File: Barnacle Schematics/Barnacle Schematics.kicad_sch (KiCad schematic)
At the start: 17 parts, among them M3 MG996, M4 SG90, SW1 Reset, U1 TiVa

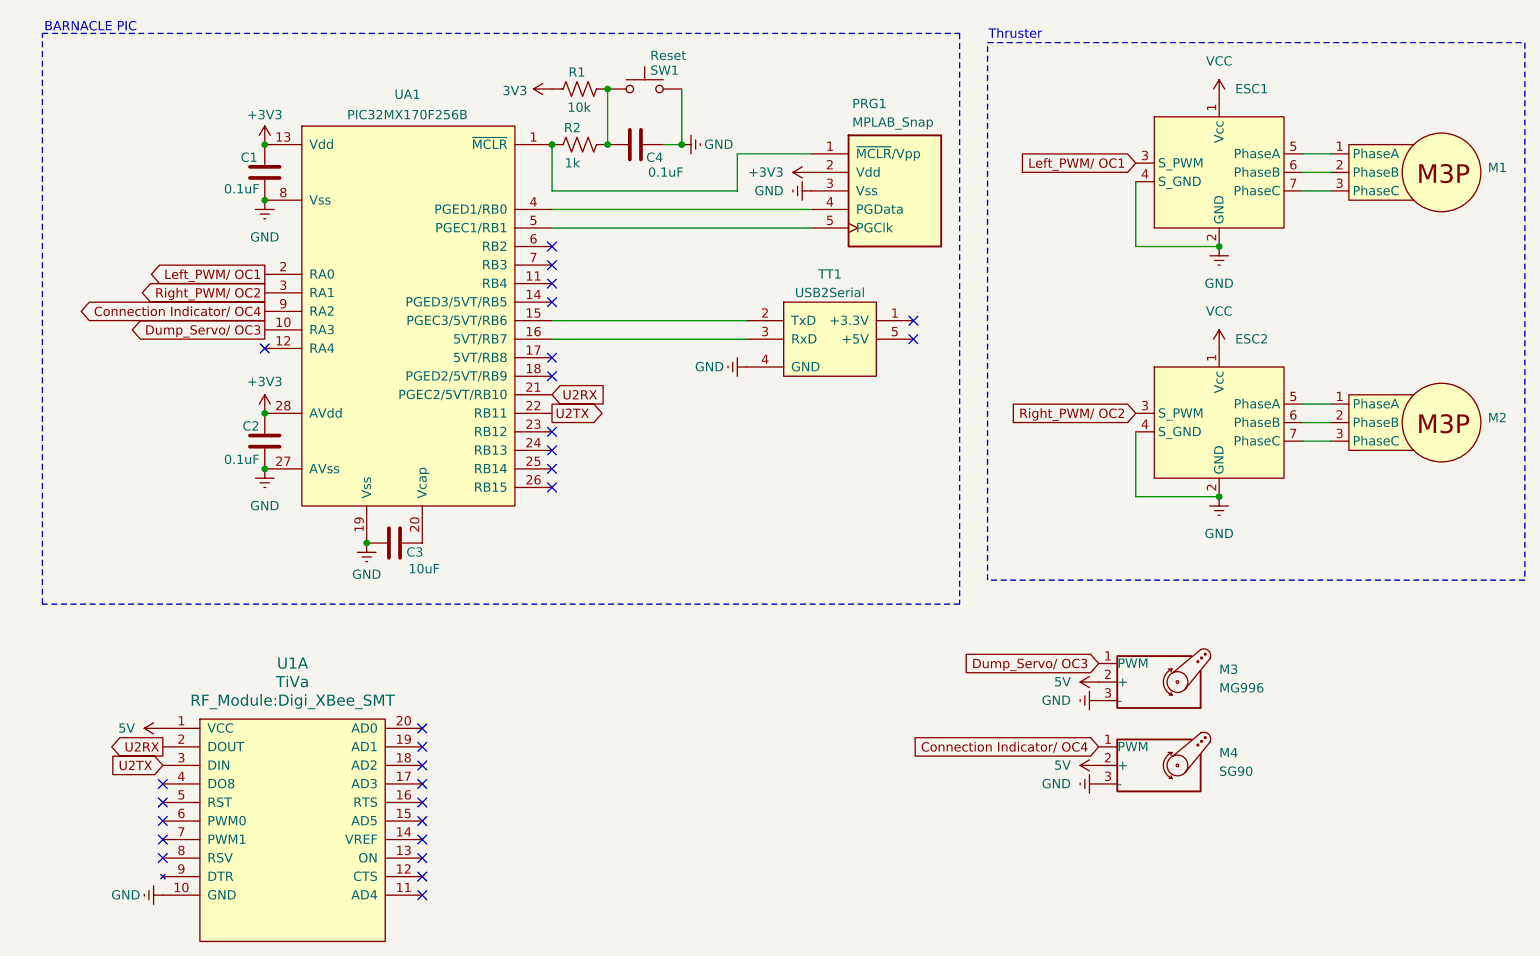
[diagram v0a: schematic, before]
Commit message: try merge with main after final
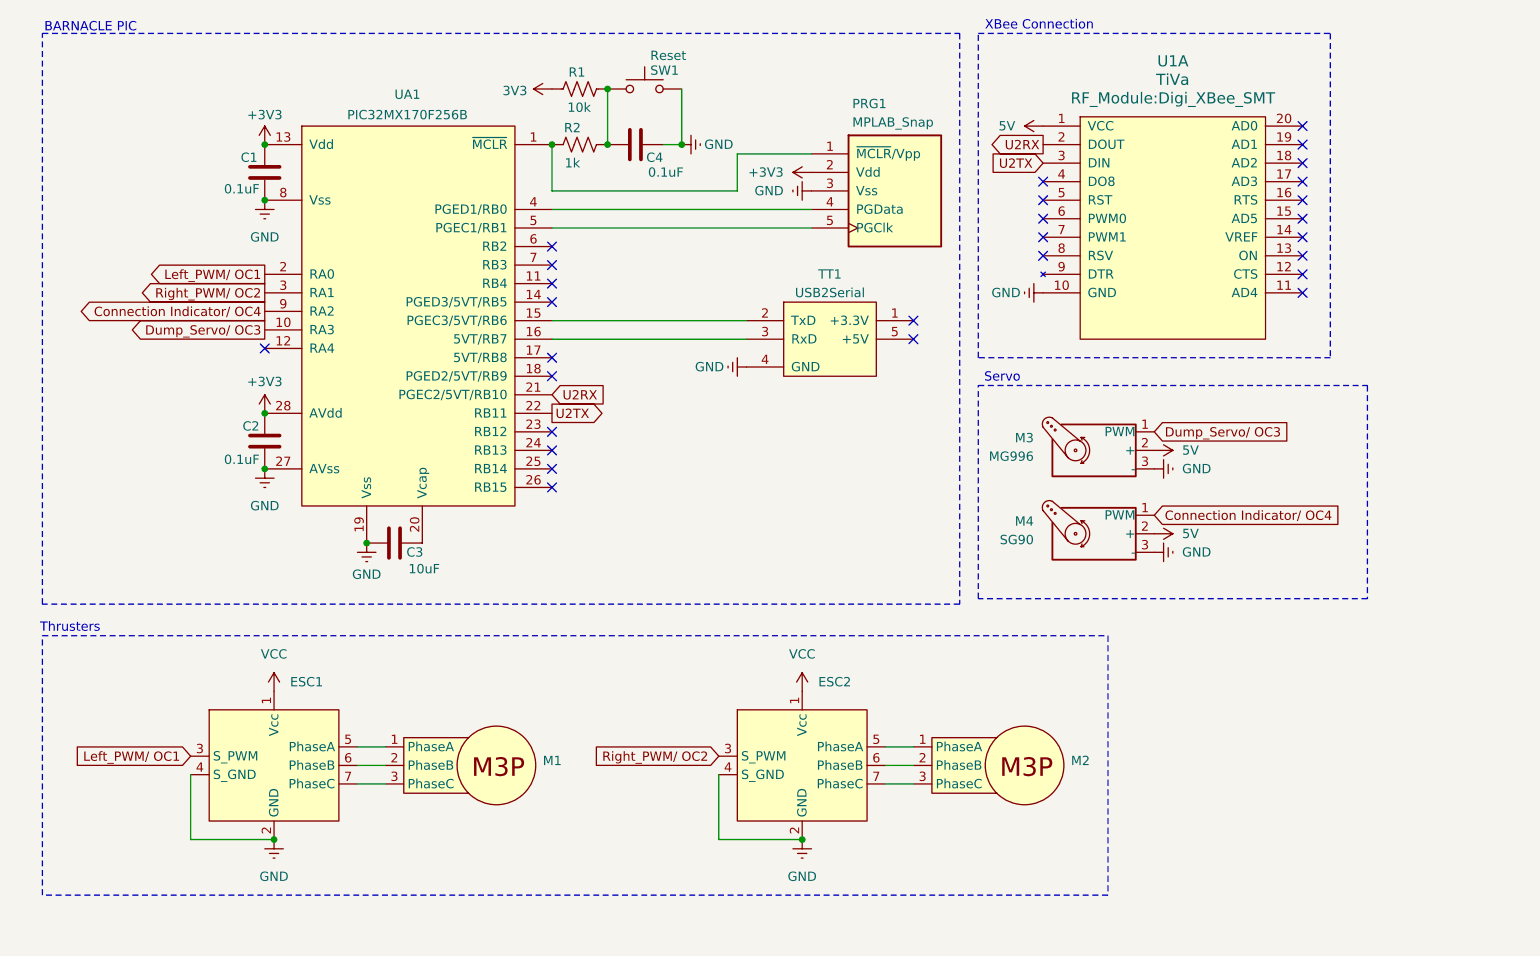
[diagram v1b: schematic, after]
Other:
- note added: "Servo"
- note added: "Thrusters"
- note added: "XBee Connection"
- note removed: "Thruster"
- company: (none) -> Team 6
- title: (none) -> BARNACLE Schematics
- moved on the sheet: ESC1, ESC2, M1, M2, M3, M4, U1A
